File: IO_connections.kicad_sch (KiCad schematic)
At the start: 8 parts, among them J1 LCD_Conn, J2 XT60 - M, J3 IMU_FFC_Conn, J4 JTAG_Conn, J5 IR_LED, J6 IR_SENSOR, J7 ESC_Conn

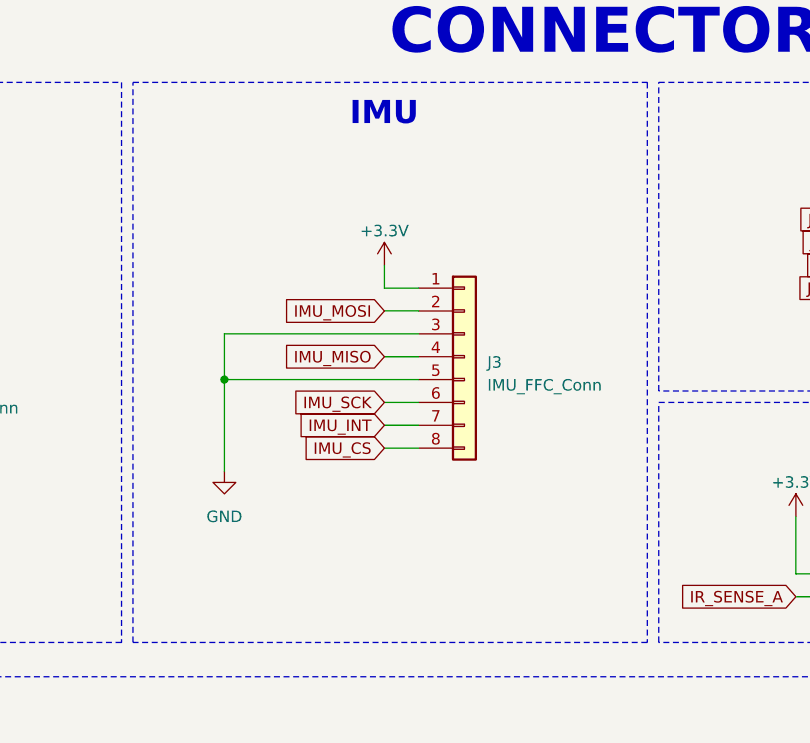
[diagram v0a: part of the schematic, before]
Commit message: Divided project
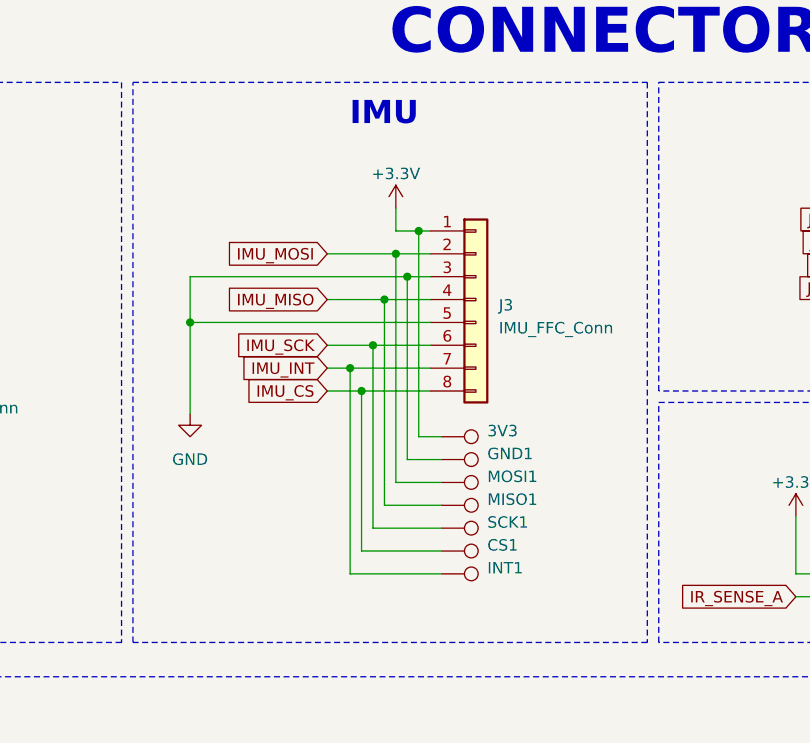
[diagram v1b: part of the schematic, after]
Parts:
- added 3V3, CS1, GND1, INT1, MISO1, MOSI1, SCK1: ~, TestPoint:TestPoint_Pad_D2.0mm, symbol Connector:TestPoint
- J2: footprint Connector_AMASS:AMASS_XT60PW-M_1x02_P7.20mm_Horizontal -> Library:XT60-SURF
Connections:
- net +3.3V: now also 3V3.1
- net GND: now also GND1.1
- net IMU_CS: now also CS1.1
- net IMU_INT: now also INT1.1
- net IMU_MISO: now also MISO1.1
- net IMU_MOSI: now also MOSI1.1
- net IMU_SCK: now also SCK1.1
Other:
- moved on the sheet: J3
